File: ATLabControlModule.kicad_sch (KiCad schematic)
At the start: 7 parts, among them J1 USB_Type_C_Receptacle, U1 STM32G0B1KEUx, U2 USBLC6-2P6

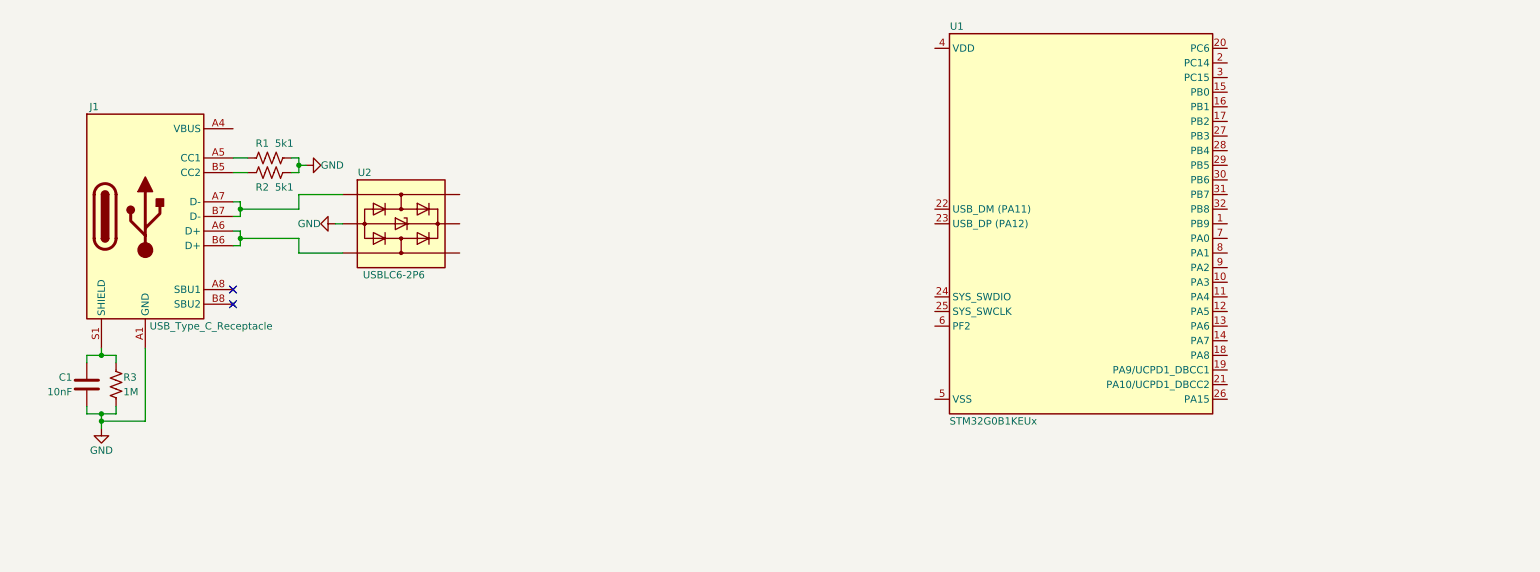
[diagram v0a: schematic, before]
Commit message: update library and schematic
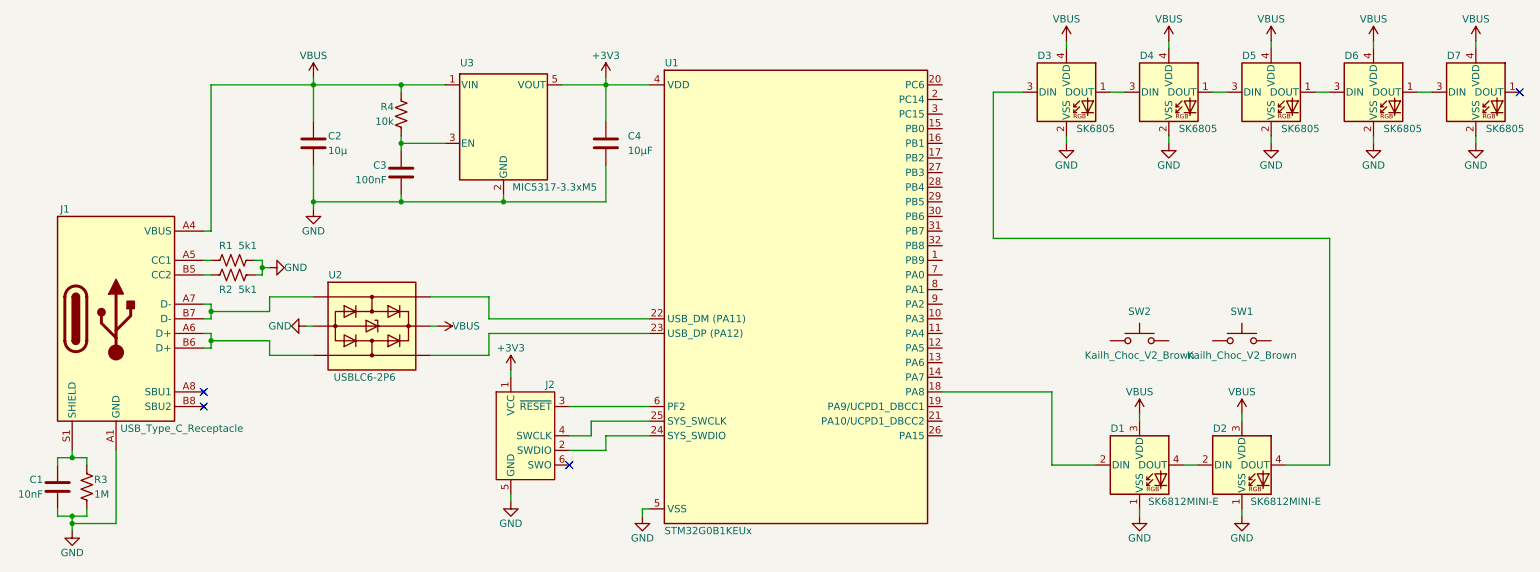
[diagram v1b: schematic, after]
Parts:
- added C2: 10µ, ATLabControlModule:C_0805_(2012_Metric), symbol ATLabControlModule:C_0805_(2012_Metric)
- added C3: 100nF, ATLabControlModule:C_0402_(1005_Metric), symbol ATLabControlModule:C_0402_(1005_Metric)
- added C4: 10µF, ATLabControlModule:C_0805_(2012_Metric), symbol ATLabControlModule:C_0805_(2012_Metric)
- added D1, D2: SK6812MINI-E, ATLabControlModule:LED_SK6812MINI-E_3.2x2.8mm_P1.5mm_ReverseMount, symbol ATLabControlModule:SK6812MINI-E
- added D3, D4, D5, D6, D7: SK6805, ATLabControlModule:LED_SK6812_EC15_1.5x1.5mm, symbol ATLabControlModule:SK6805
- added J2: Conn_ARM_SWD_TagConnect_TC2030, ATLabControlModule:Tag-Connect_TC2030-IDC-NL_2x03_P1.27mm_Vertical, symbol ATLabControlModule:Conn_ARM_SWD_TagConnect_TC2030
- added R4: 10k, ATLabControlModule:R_0402_(1005_Metric), symbol ATLabControlModule:R_0402_(1005_Metric)
- added SW1, SW2: Kailh_Choc_V2_Brown, ATLabControlModule:SW_Kailh_Choc_V2, symbol ATLabControlModule:Kailh_Choc_V2_Brown
- added U3: MIC5317-3.3xM5, ATLabControlModule:SOT-23-5, symbol ATLabControlModule:MIC5317-3.3xM5
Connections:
- net GND: now also U1.33 (VSS), U1.5 (VSS), C2.2, C3.2, C4.2, D1.1 (VSS), D2.1 (VSS), D3.2 (VSS), D4.2 (VSS), D5.2 (VSS), D6.2 (VSS), D7.2 (VSS), J2.5 (GND), U3.2 (GND)
- net VBUS: now reaches J1.A4 (VBUS), J1.A9 (VBUS), J1.B4 (VBUS), J1.B9 (VBUS)
- net VBUS: now also U2.5 (VBUS), C2.1, D1.3 (VDD), D2.3 (VDD), D3.4 (VDD), D4.4 (VDD), D5.4 (VDD), D6.4 (VDD), D7.4 (VDD), R4.1, U3.1 (VIN)
- net at U2.4 (I/O2): now also U1.23 (PA10/PA12)
- net at U2.6 (I/O1): now also U1.22 (PA9/PA11)
- net at U1.18 (PA8): now also D1.2 (DIN)
- net at U1.24 (PA13): now also J2.2 (SWDIO)
- net at U1.25 (PA14): now also J2.4 (SWCLK)
- net +3V3: now reaches U1.4 (VDD)
- net +3V3: now also C4.1, J2.1 (VCC), U3.5 (VOUT)
- net at U1.6 (PF2): now also J2.3 (~{RESET})
- new net: D6.1 (DOUT), D7.3 (DIN)
- new net: D5.1 (DOUT), D6.3 (DIN)
- new net: C3.1, R4.2, U3.3 (EN)
- new net: D4.1 (DOUT), D5.3 (DIN)
- new net: D3.1 (DOUT), D4.3 (DIN)
- new net: D2.4 (DOUT), D3.3 (DIN)
- new net: D1.4 (DOUT), D2.2 (DIN)
- no-connect marks 2 -> 4
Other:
- moved on the sheet: C1, J1, R1, R2, R3, U1, U2
